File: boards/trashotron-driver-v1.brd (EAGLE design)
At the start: 82.5 x 63.5 mm, 11 parts, among them IC1 2967-MP6500, IC2 2967-MP6500, IC3 2967-MP6500, J2 455-1750-1-ND, J4 455-1750-1-ND, J6 455-1750-1-ND

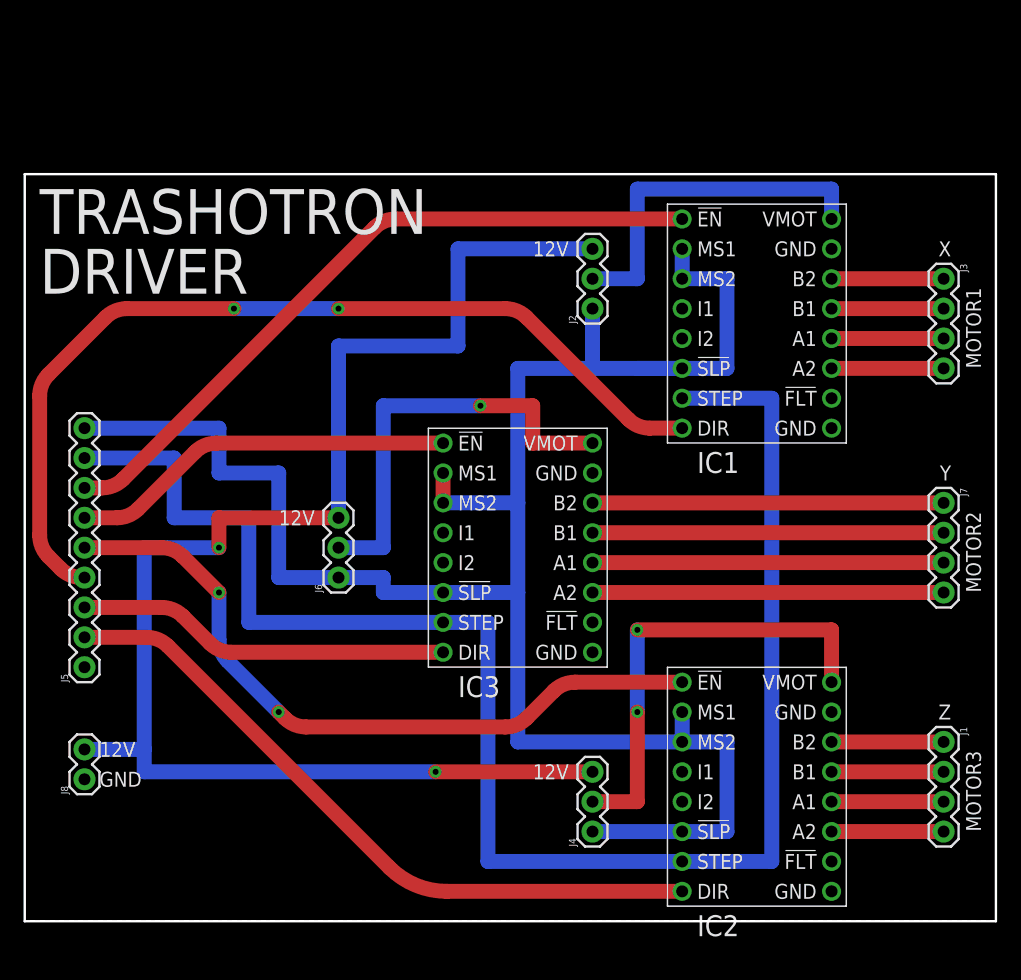
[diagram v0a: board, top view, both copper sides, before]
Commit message: lots of work on pcb layout
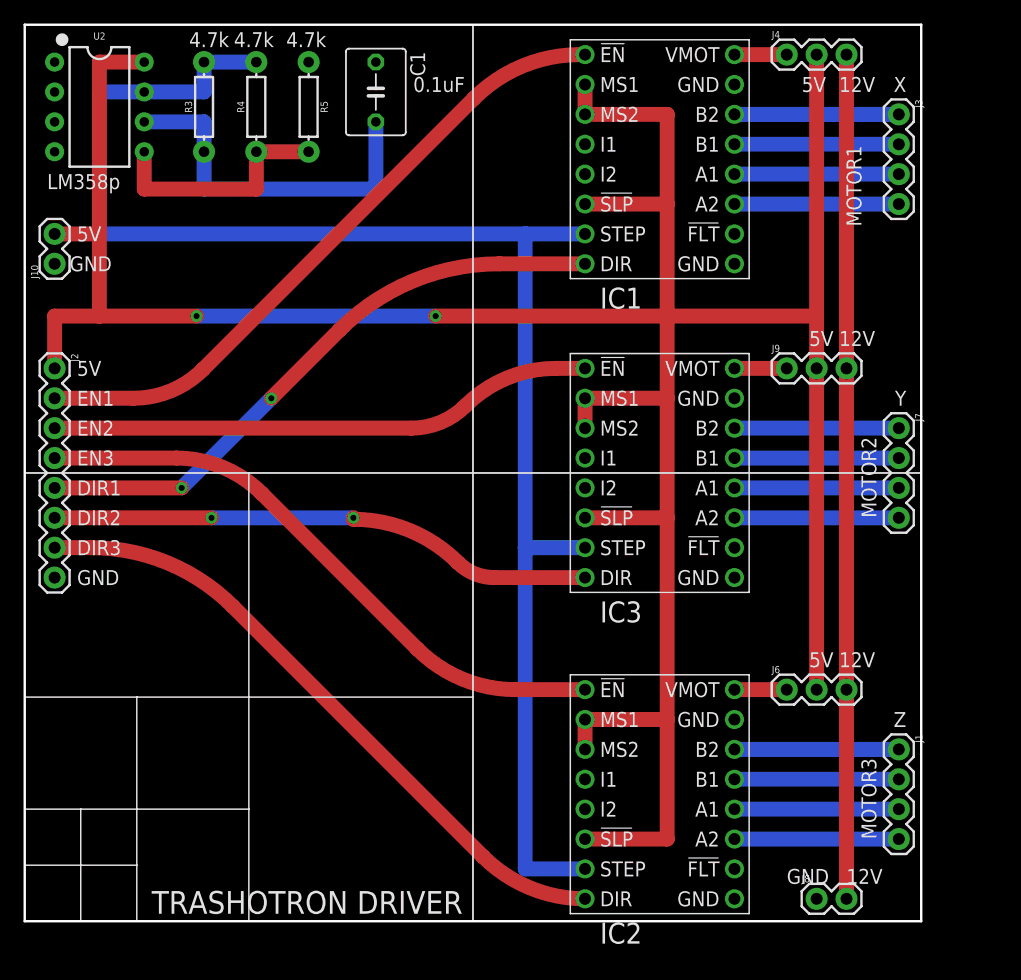
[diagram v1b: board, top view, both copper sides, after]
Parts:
- removed J5: (no value), SparkFun-Connectors:1X09
- added C1: (no value), rcl:C050-050X075
- added J10: (no value), SparkFun-Connectors:1X02
- added J9: 455-1750-1-ND, SparkFun-Connectors:1X03
- added R3, R4, R5: (no value), SparkFun-Resistors:AXIAL-0.3
- added U2: LM358, SparkFun-IC-Amplifiers:DIP08
- J2: value 455-1750-1-ND -> (none); device SparkFun-Connectors:1X03 -> SparkFun-Connectors:1X08
- moved J4 68.1 mm to (64.8, 73.7), turned to 0 degrees
- moved J8 63.1 mm to (67.3, 1.91), turned to 0 degrees
- moved J2 46.0 mm to (2.54, 47.0), turned to 270 degrees
- moved J6 39.3 mm to (64.8, 19.7), turned to 0 degrees
- moved IC1 16.2 mm to (54.0, 64.8)
- moved J3 14.5 mm to (74.3, 68.6)
- moved IC3 13.6 mm to (54.0, 38.1)
- moved IC2 8.28 mm to (54.0, 10.8)
- moved J7 7.41 mm to (74.3, 41.9)
- moved J1 3.86 mm to (74.3, 14.6)
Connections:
- new net N$18: C1.2, R3.P$1, U2.6
- new net N$19: R4.P$1, R5.P$2, U2.5
- net 5V: now also J10.2, J4.2, J6.2, J9.2, U2.8; no longer J4.1, J5.9, J6.1
- net CLOCK: now also R3.P$2, R4.P$2, U2.7; no longer J5.8
- net DIR1: now also J2.5; no longer J5.4
- net DIR2: now also J2.6; no longer J5.3
- net DIR3: now also J2.7; no longer J5.2
- net EN1: now also J2.2; no longer J5.7
- net EN2: now also J2.3; no longer J5.6
- net EN3: now also J2.4; no longer J5.5
- net EXTPOW: now also J9.3; no longer J2.3
- net GND: now also C1.1, J10.1, J2.8, R5.P$1, U2.4; no longer J5.1
- net VMOT1: now also J4.1; no longer J2.2
- net VMOT2: now also J9.1; no longer J6.2
- net VMOT3: now also J6.1; no longer J4.2
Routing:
- net 5V: track 171.4 -> 263.5 mm, vias 0 -> 2
- net EXTPOW: track 125.7 -> 71.8 mm, vias 2 -> 0
- net VMOT3: track 39.4 -> 4.44 mm, vias 2 -> 0
- net VMOT2: track 36.8 -> 4.44 mm, vias 1 -> 0
- net N$18: track 0.00 -> 31.1 mm
- net DIR1: track 79.3 -> 51.8 mm
- net VMOT1: track 30.5 -> 4.44 mm
- net N$19: track 0.00 -> 20.3 mm
- net N$4: track 29.8 -> 14.0 mm
- net N$14: track 29.8 -> 14.0 mm
- net N$13: track 29.8 -> 14.0 mm
- net N$1: track 29.8 -> 14.0 mm
- net DIR2: track 31.7 -> 46.2 mm, vias 0 -> 2
- net EN2: track 32.8 -> 46.1 mm
- net EN3: track 60.9 -> 51.8 mm, vias 2 -> 0
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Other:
- board size 82.5 x 63.5 mm -> 76.2 x 76.2 mm
- board text added: "0.1uF"
- board text added: "4.7k"
- board text added: "5V"
- board text added: "DIR1"
- board text added: "DIR2"
- board text added: "DIR3"
- board text added: "EN1"
- board text added: "EN2"
- board text added: "EN3"
- board text added: "LM358p"
- board text added: "TRASHOTRON DRIVER"
- board text removed: "DRIVER"
- board text removed: "TRASHOTRON"
